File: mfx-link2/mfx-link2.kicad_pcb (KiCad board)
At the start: 2 copper layers, 50 x 50 mm, 60 parts, among them P1 CONN_01X04, P2 Gleisbox, P4 UART, P5 I2C, P6 CONN_02X03, P7 POTI, P8 IBT-2, Q1 BC817-40, SW1 SW_PUSH, T1 53040C, U1 6N137, U2 7805, U3 LM393, U4 78L05, U5 PIC16F1709

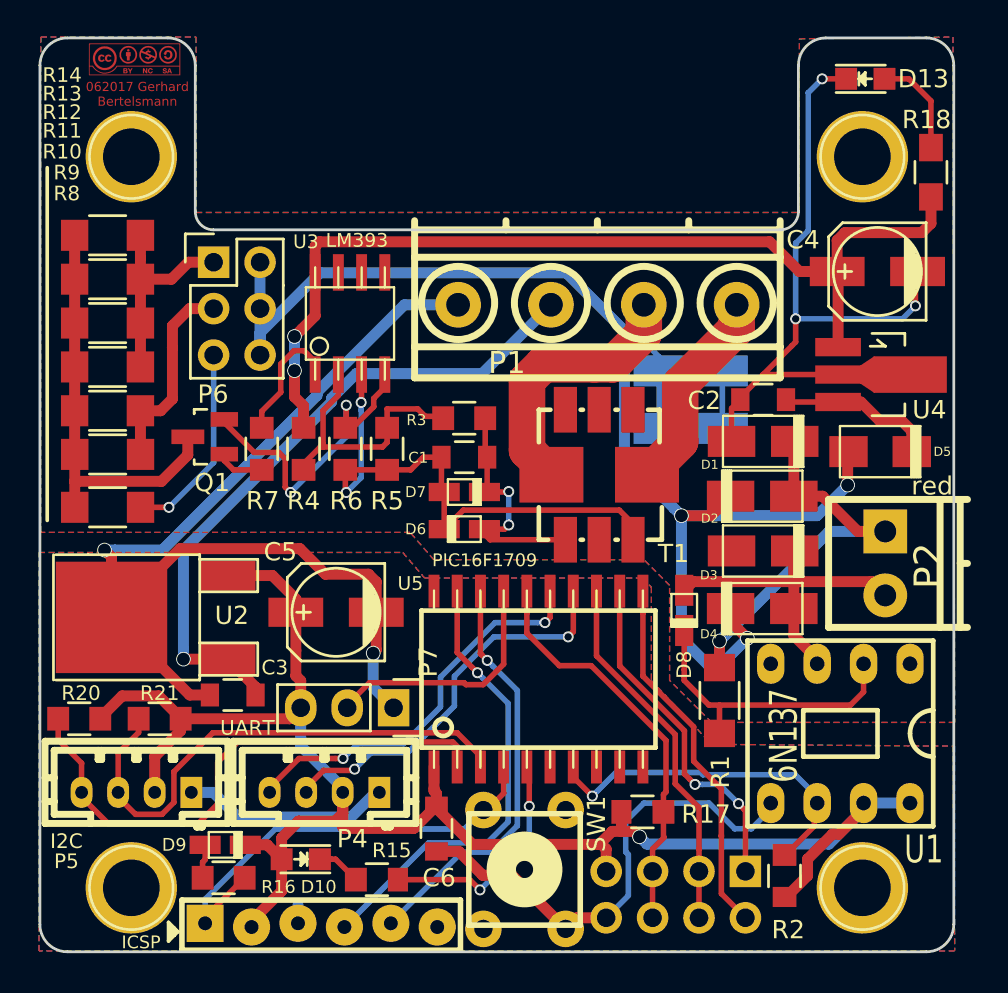
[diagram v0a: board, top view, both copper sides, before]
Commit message: production
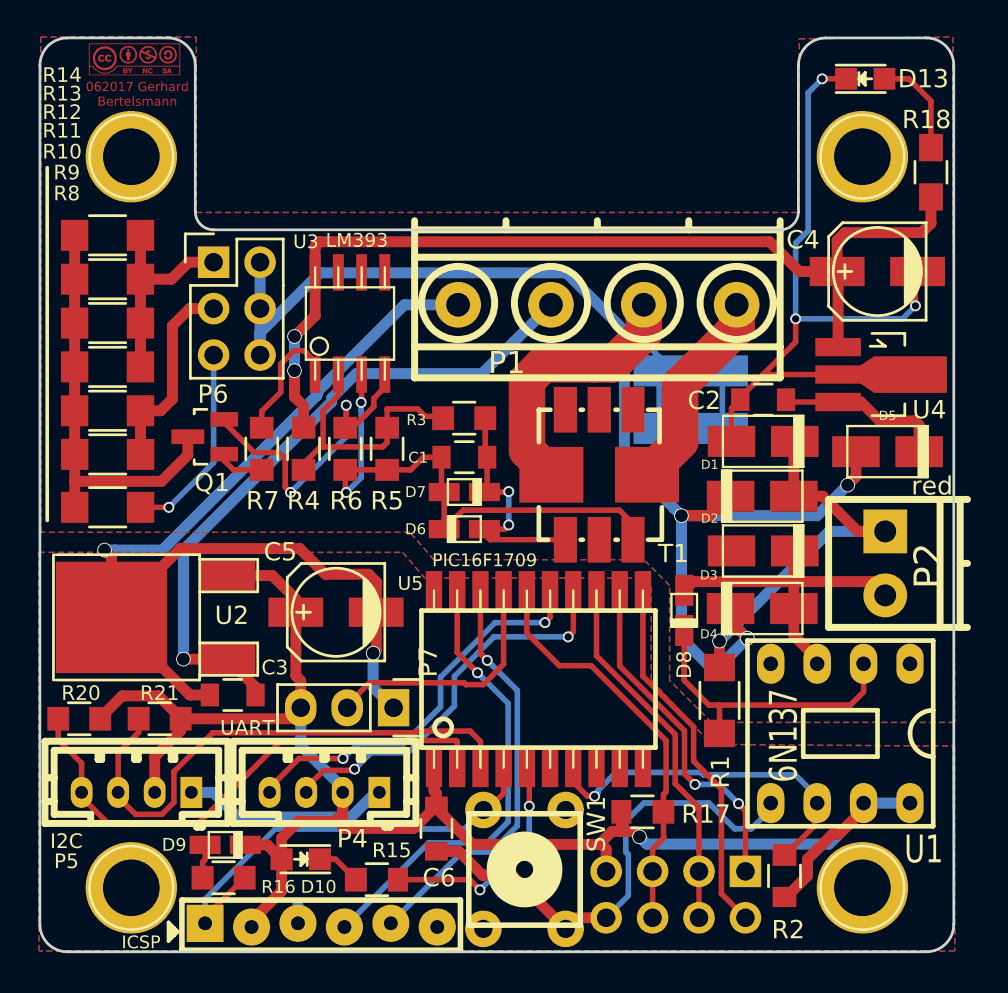
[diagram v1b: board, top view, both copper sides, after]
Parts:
- moved D5 0.41 mm to (166.8, 116.5)
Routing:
- net /SDA: track 28.9 -> 30.1 mm
- net /SCL: track 31.0 -> 29.9 mm
- net /PULSE: track 19.6 -> 20.4 mm
- net /VI: track 9.87 -> 10.5 mm
